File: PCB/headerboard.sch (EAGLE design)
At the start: 11 parts

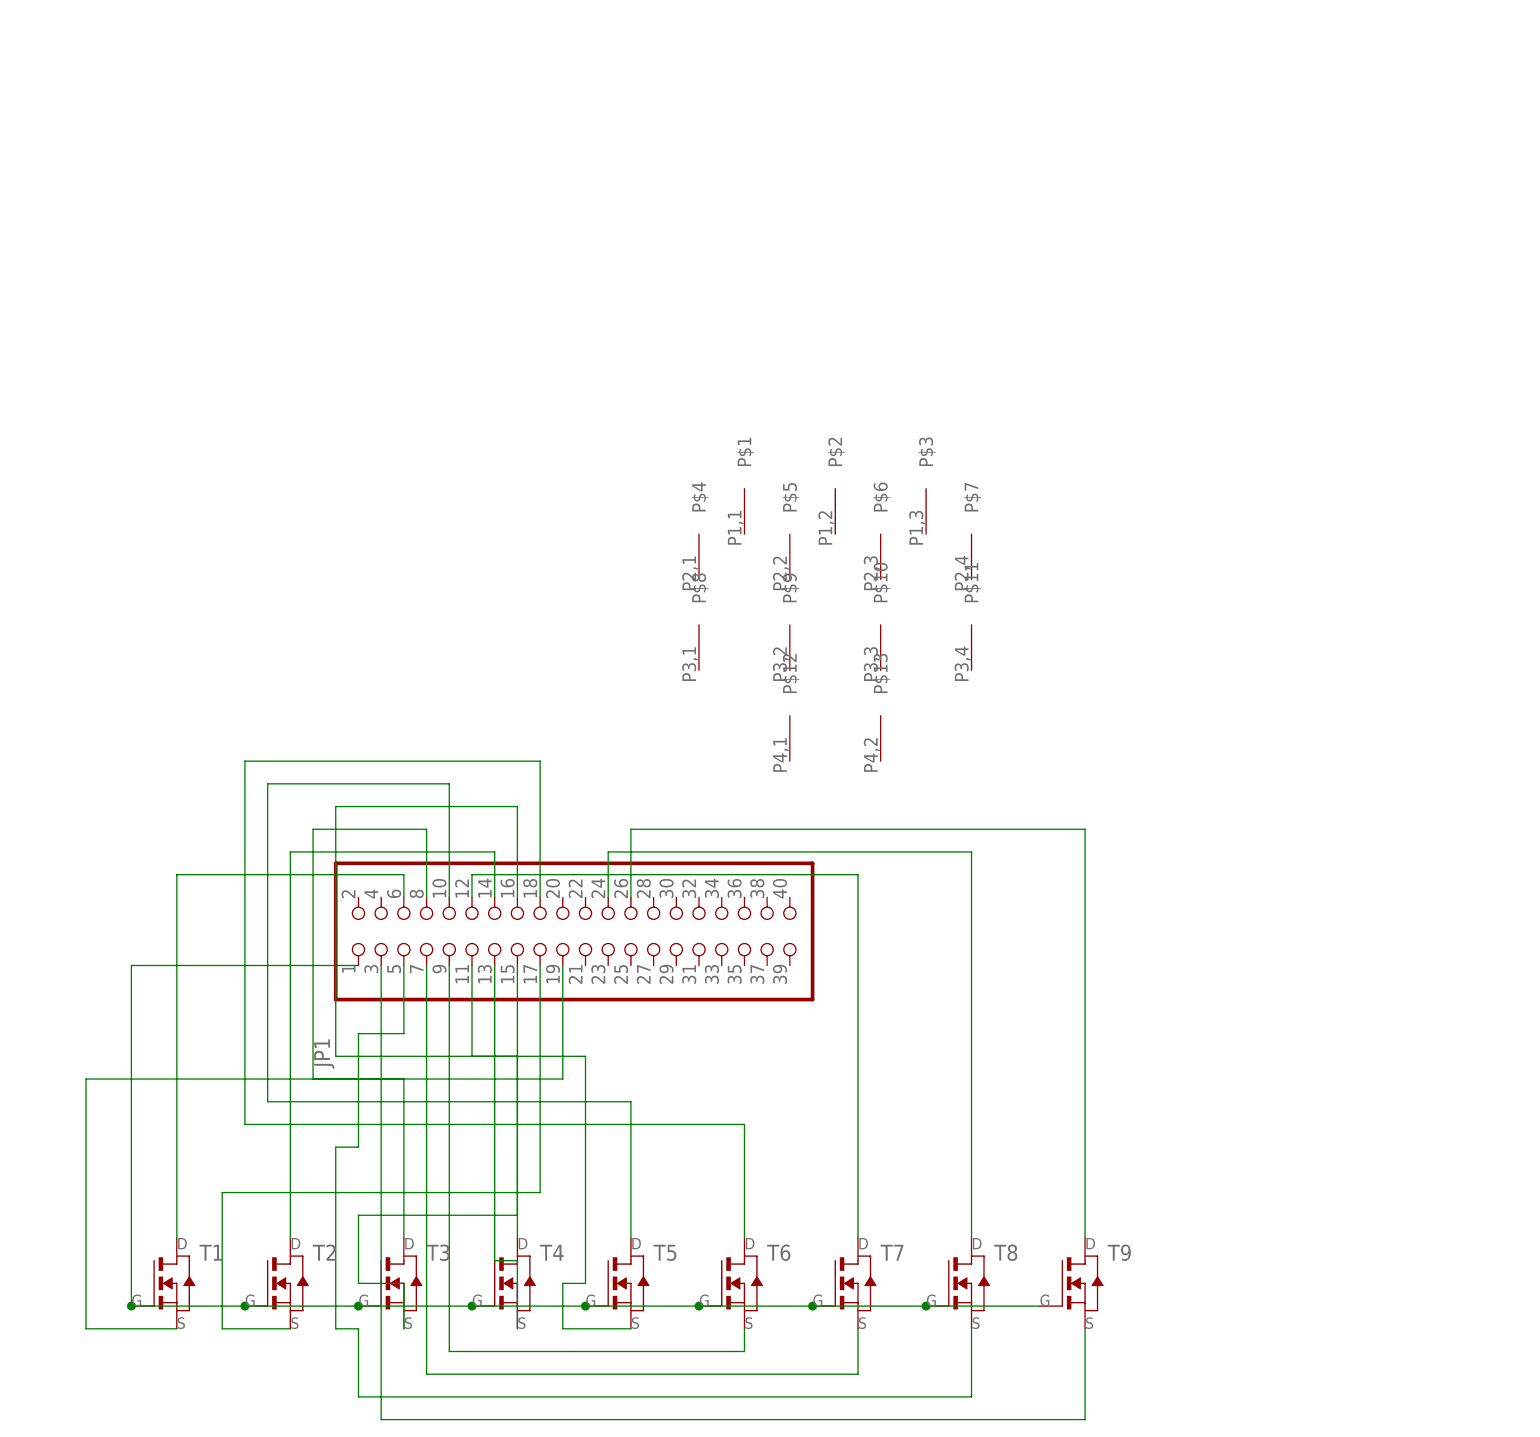
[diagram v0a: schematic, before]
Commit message: header board and schematic
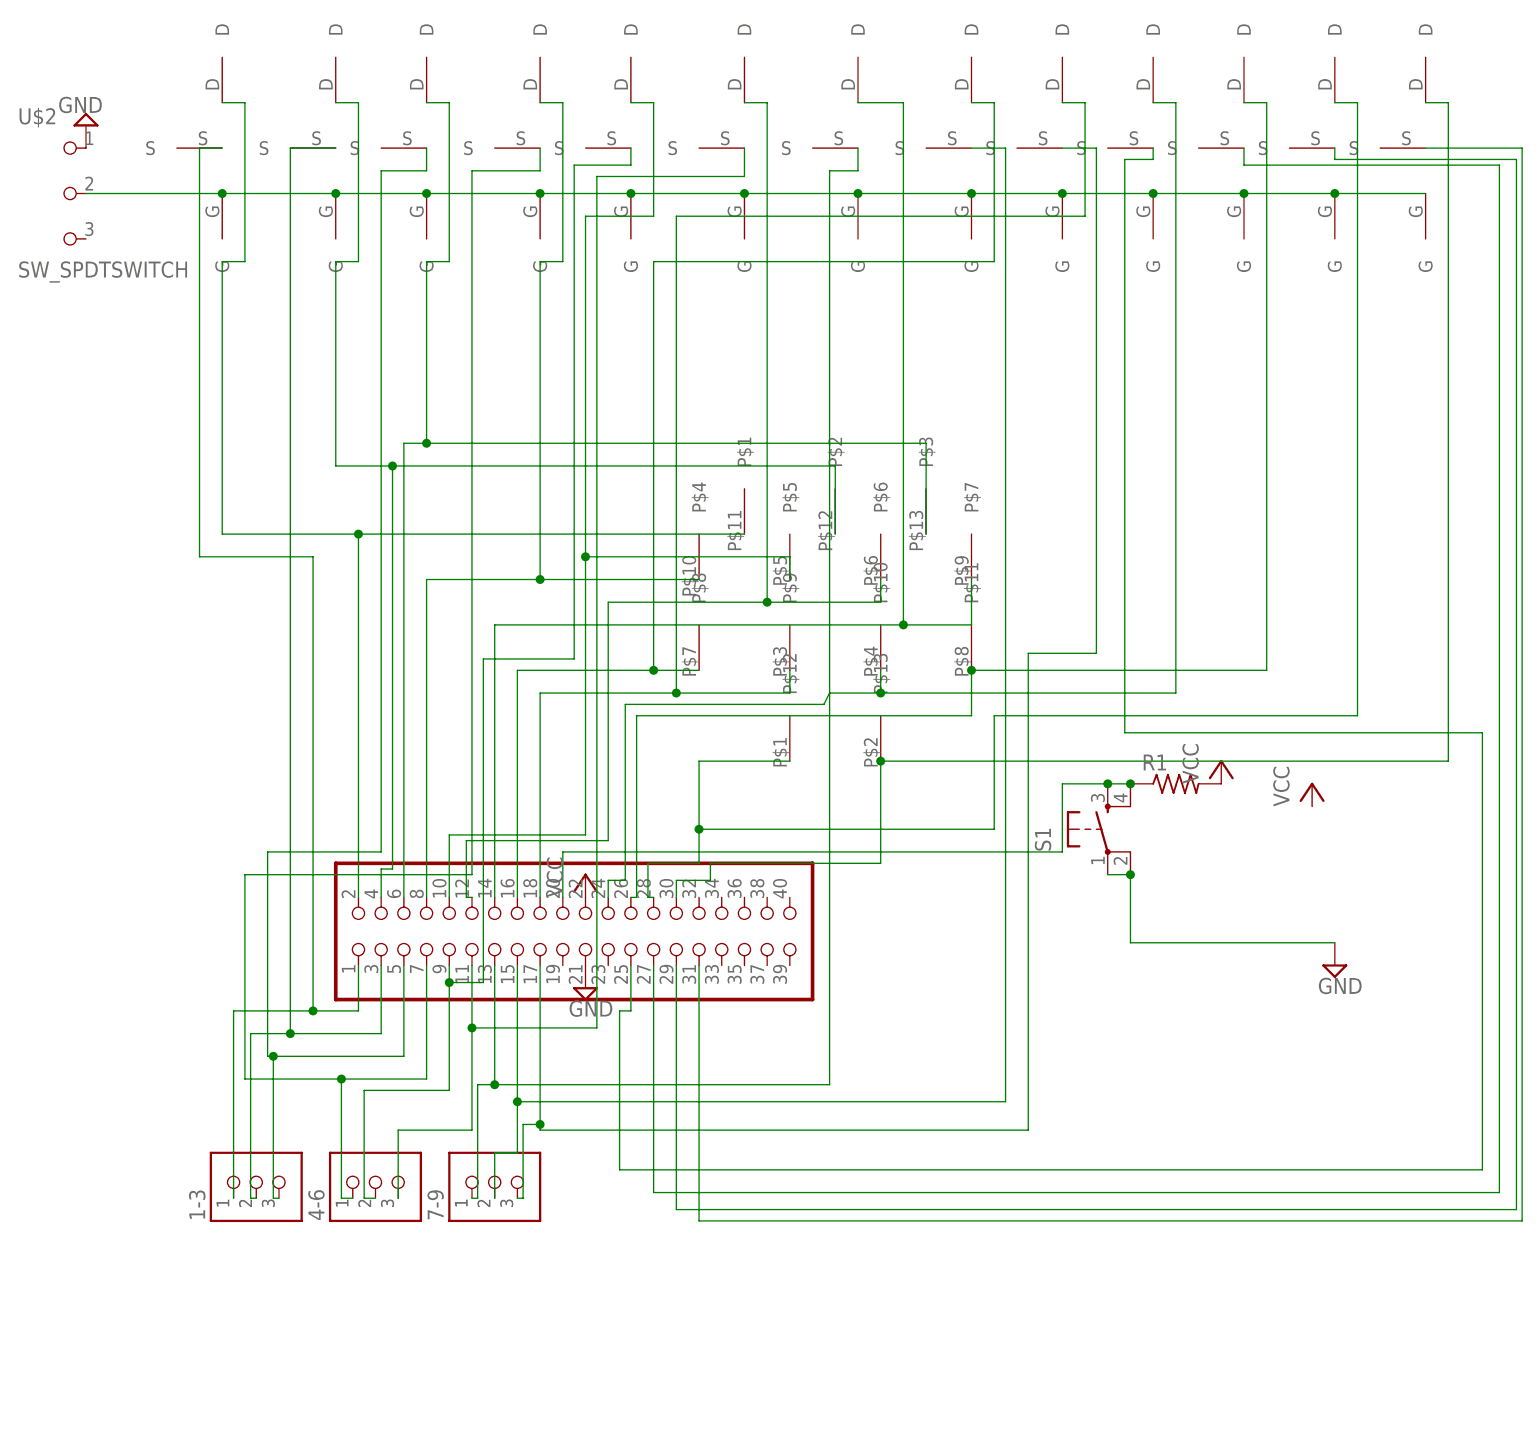
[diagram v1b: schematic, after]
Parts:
- removed T1, T2, T3, T4, T5, T6, T7, T8, T9: (no value), eagle_fab:MOSFET_NSOT23
- added 1-3, 4-6, 7-9: CONN_03_TERM'-FABLAB', fab_new:CONN_03_TERM'-FABLAB'
- added R1: (no value), fab_new:R1206FAB
- added S1: (no value), fab_new:SW_SWITCH_TACTILE_6MM6MM_SWITCH
- added U$10, U$11, U$12, U$13, U$14, U$15, U$3, U$4, U$5, U$6, U$7, U$8, U$9: SOT23NMOS, ContunityTestingRig:SOT23NMOS
- added U$2: SW_SPDTSWITCH, fab_new:SW_SPDTSWITCH
- renumbered U$1 to U$19
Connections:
- new net GND: JP1.21, S1.P, S1.P1, U$2.1
- new net N$20: 7-9.1, JP1.13, U$9.S
- new net N$21: JP1.10, U$19.P$5, U$7.D
- new net N$22: 7-9.2, JP1.15, U$10.S
- new net N$23: 7-9.3, JP1.17, U$11.S
- new net N$24: JP1.25, U$12.S
- new net N$25: JP1.27, U$13.S
- new net N$26: JP1.29, U$14.S
- new net N$27: JP1.31, U$15.S
- new net N$37: 1-3.1, JP1.1, U$3.S
- new net VCC: JP1.22, R1.2
- net N$1: now also U$10.G, U$11.G, U$12.G, U$13.G, U$14.G, U$15.G, U$2.2, U$3.G, U$4.G, U$5.G, U$6.G, U$7.G, U$8.G, U$9.G; no longer JP1.1, T1.G, T2.G, T3.G, T4.G, T5.G, T6.G, T7.G, T8.G, T9.G
- net N$10: now also JP1.18, U$11.D, U$19.P$9; no longer JP1.26, T9.D
- net N$11: now also 1-3.2, JP1.3, U$4.S; no longer JP1.19, T1.S
- net N$12: now also JP1.28, U$14.D, U$19.P$12; no longer JP1.17, T2.S
- net N$13: now also JP1.24, U$12.D, U$19.P$10; no longer JP1.15, T3.S
- net N$14: now also JP1.30, U$15.D, U$19.P$13; no longer JP1.13, T4.S
- net N$15: now also 1-3.3, JP1.5, U$5.S; no longer JP1.11, T5.S
- net N$16: now also JP1.20, R1.1, S1.S, S1.S1; no longer JP1.9, T6.S
- net N$17: now also 4-6.1, U$6.S; no longer T7.S
- net N$18: now also 4-6.2, JP1.9, U$7.S; no longer JP1.5, T8.S
- net N$19: now also 4-6.3, JP1.11, U$8.S; no longer JP1.3, T9.S
- net N$2: now also JP1.2, U$19.P$1, U$3.D; no longer JP1.6, T1.D
- net N$3: now also JP1.4, U$19.P$2, U$4.D; no longer JP1.14, T2.D
- net N$4: now also JP1.6, U$19.P$3, U$5.D; no longer JP1.8, T3.D
- net N$5: now also JP1.8, U$19.P$4, U$6.D; no longer JP1.16, T4.D
- net N$6: now also JP1.12, U$19.P$6, U$8.D; no longer JP1.10, T5.D
- net N$7: now also JP1.26, U$13.D, U$19.P$11; no longer JP1.18, T6.D
- net N$8: now also JP1.14, U$19.P$7, U$9.D; no longer JP1.12, T7.D
- net N$9: now also JP1.16, U$10.D, U$19.P$8; no longer JP1.24, T8.D
